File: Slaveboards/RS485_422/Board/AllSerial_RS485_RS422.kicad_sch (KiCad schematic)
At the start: 18 parts, among them IC1 7402D, IC2 MAX485CSA, IC3 MAX485CSA, IC4 MAX485CSA, IC5 MAX485CSA, J1 PinHeader_2x05_P2.54mm_Horizo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, X1 ALLSERIALSLAVE, X2 AKL18X-10W

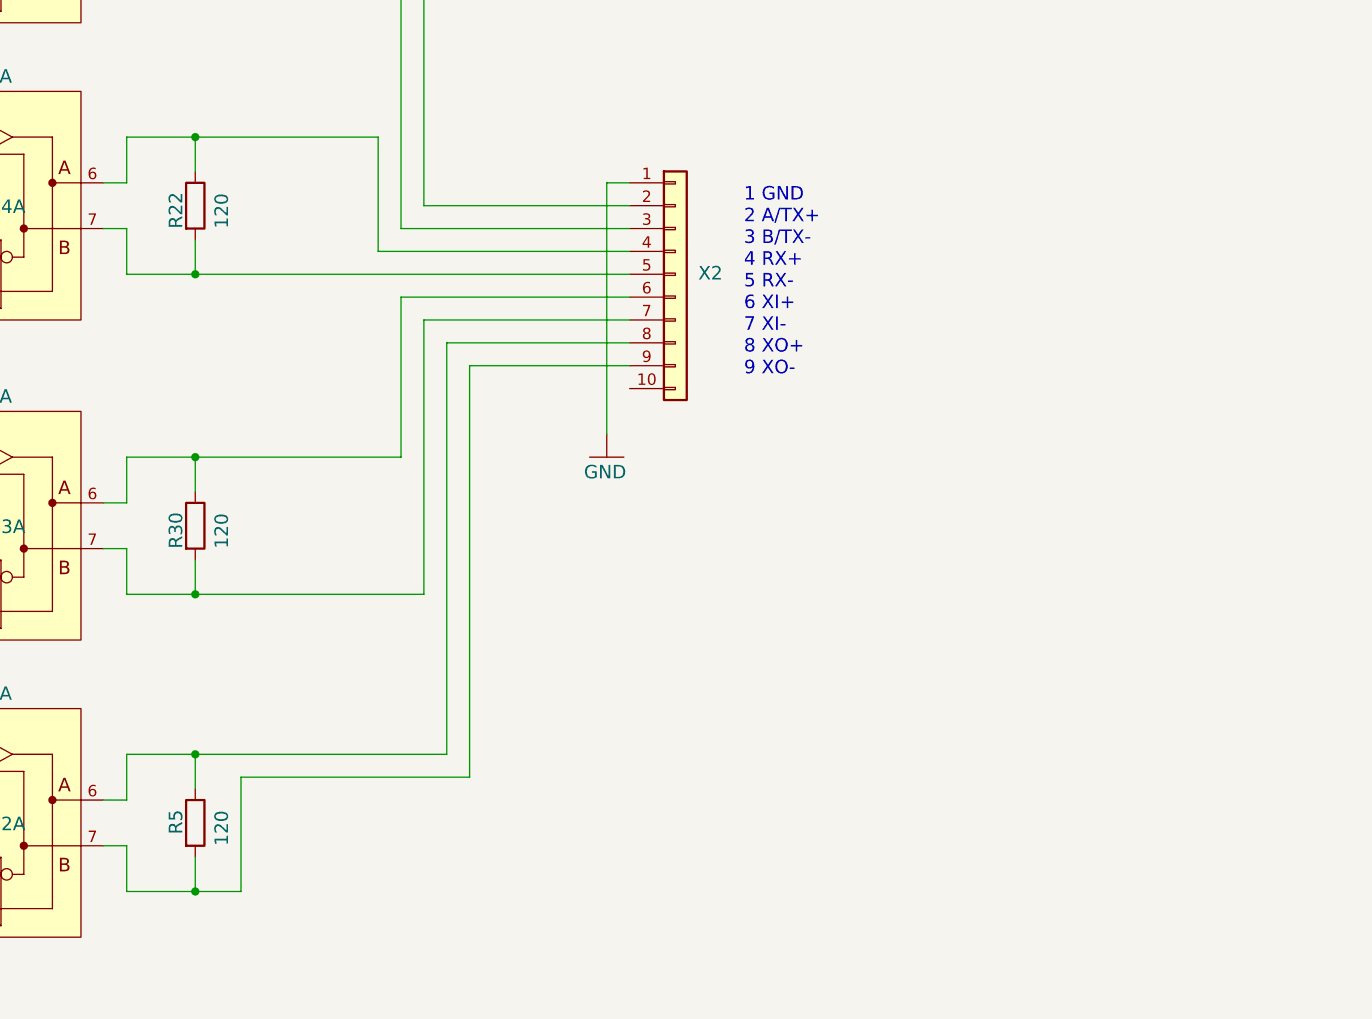
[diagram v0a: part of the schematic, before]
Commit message: Improve libraries
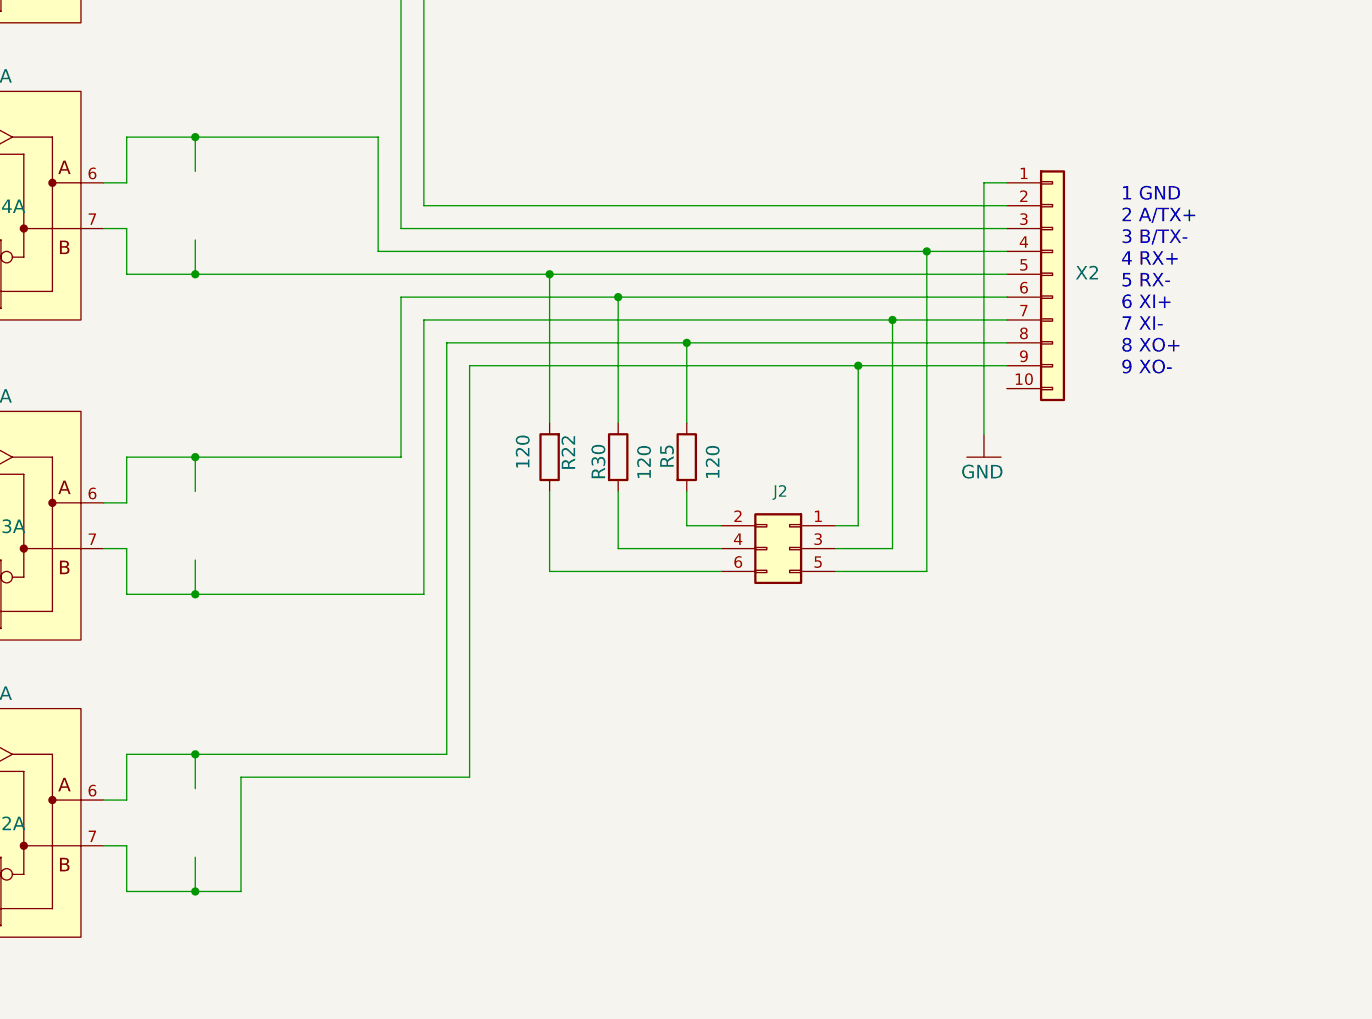
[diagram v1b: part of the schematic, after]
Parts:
- added J2: Conn_02x03_Odd_Even, Connector_PinHeader_2.54mm:PinHeader_2x03_P2.54mm_Vertical, symbol Connector_Generic:Conn_02x03_Odd_Even
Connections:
- net at IC4.6 (A), X2.4 (Pin_4): now also J2.5 (Pin_5); no longer R22.1
- net at IC3.7 (B), X2.7 (Pin_7): now also J2.3 (Pin_3); no longer R30.2
- net at IC2.7 (B), X2.9 (Pin_9): now also J2.1 (Pin_1); no longer R5.2
- new net: J2.4 (Pin_4), R30.2
- new net: J2.6 (Pin_6), R22.1
- new net: J2.2 (Pin_2), R5.2
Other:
- moved on the sheet: R22, R30, R5, X2
